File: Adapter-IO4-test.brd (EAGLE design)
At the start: 22 parts, among them CON1 CONNECTOR-IO4INV

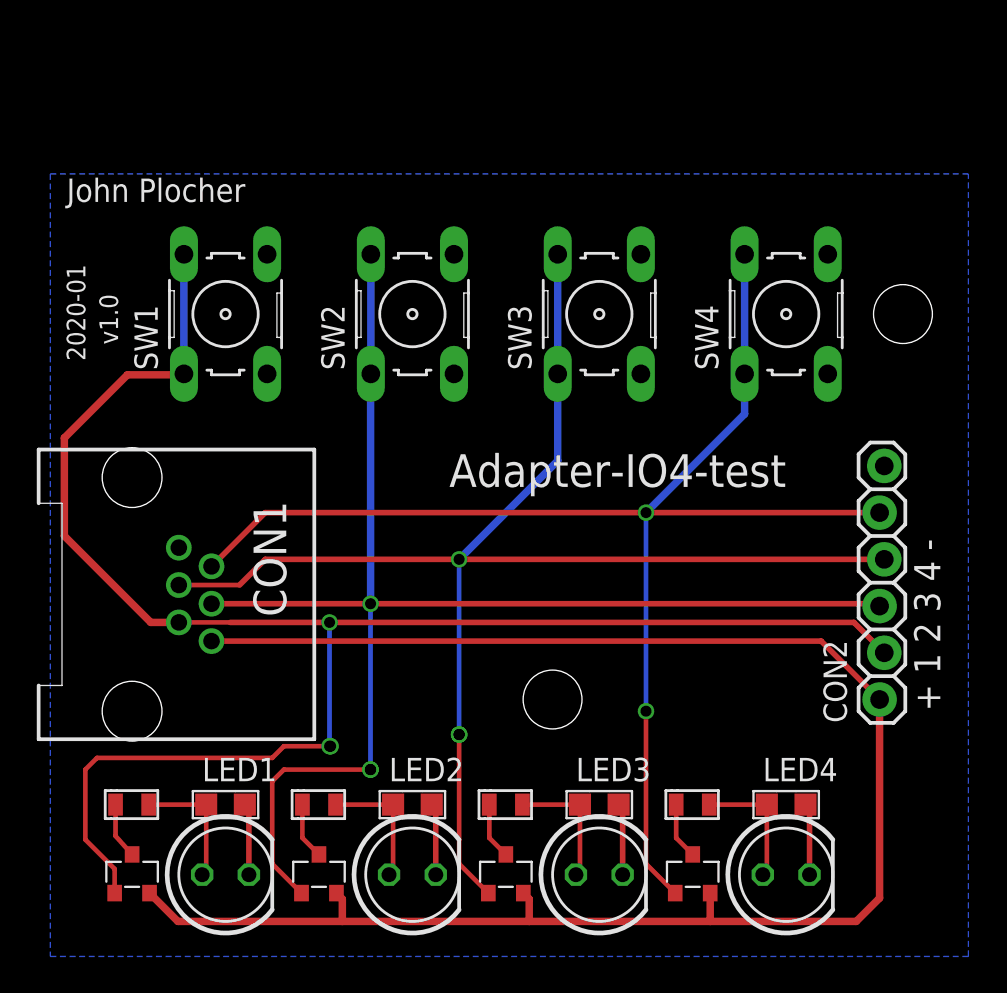
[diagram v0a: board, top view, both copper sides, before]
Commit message: simplified design
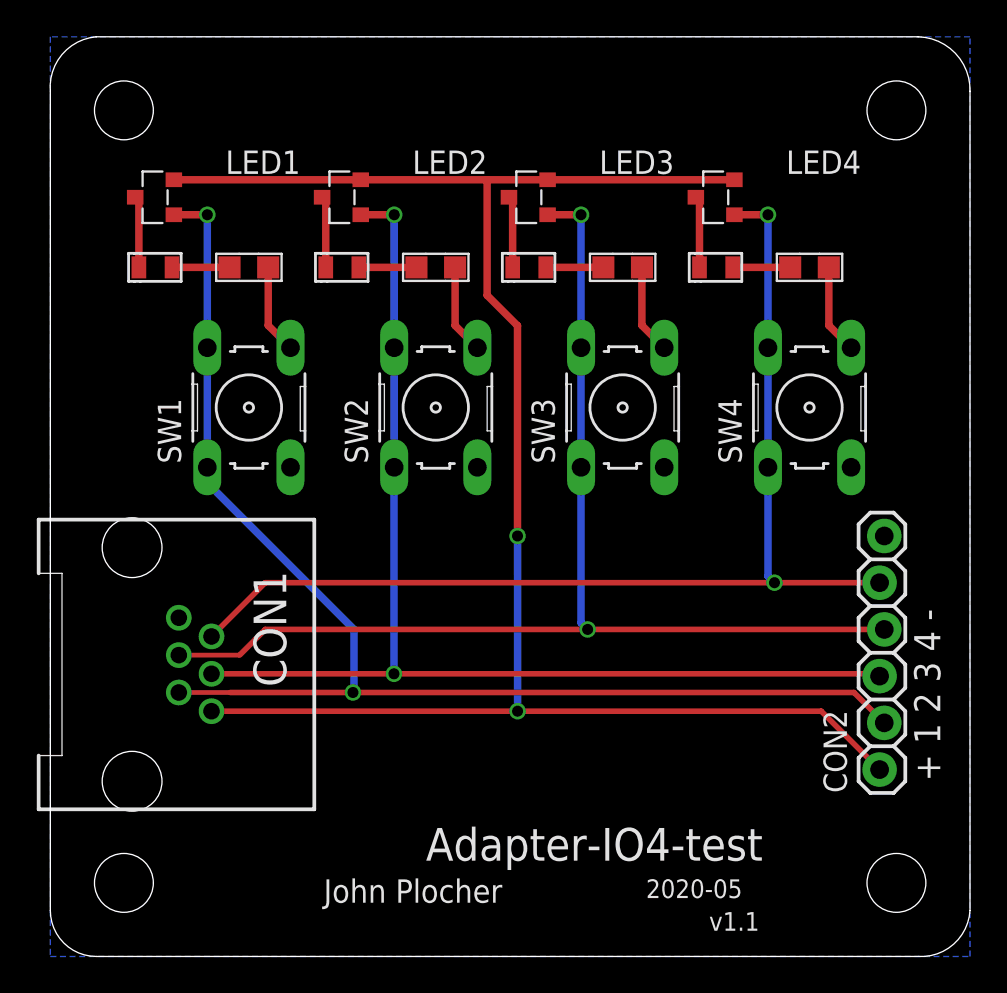
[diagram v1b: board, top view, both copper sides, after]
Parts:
- removed LED5, LED6, LED7, LED8: (no value), SPCoast:LED5MM
- added BOARD1: BOARD50X50-NOHOLES, SPCoast:BOARD-SEEED5X5-NOHOLES
- moved Q1 36.9 mm to (5.71, 41.3), turned to 90 degrees
- moved Q2 36.9 mm to (15.9, 41.3), turned to 90 degrees
- moved Q3 36.9 mm to (26.0, 41.3), turned to 90 degrees
- moved Q4 36.9 mm to (36.2, 41.3), turned to 90 degrees
- moved LED1 29.2 mm to (10.8, 37.5)
- moved LED2 29.2 mm to (21.0, 37.5)
- moved LED3 29.2 mm to (31.1, 37.5)
- moved LED4 29.2 mm to (41.3, 37.5)
- moved R1 29.2 mm to (5.71, 37.5)
- moved R2 29.2 mm to (15.9, 37.5)
- moved R3 29.2 mm to (26.0, 37.5)
- moved R4 29.2 mm to (36.2, 37.5)
- moved SW1 5.24 mm to (10.8, 29.8)
- moved SW2 5.24 mm to (21.0, 29.8)
- moved SW3 5.24 mm to (31.1, 29.8)
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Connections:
- net GND: no longer LED5.K, LED6.K, LED7.K, LED8.K
- net N$16: no longer LED8.A
- net N$2: no longer LED5.A
- net N$4: no longer LED6.A
- net N$6: no longer LED7.A
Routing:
- net N$7: track 95.0 -> 70.2 mm
- net N$10: track 75.1 -> 59.5 mm
- net N$8: track 76.7 -> 63.1 mm, vias 3 -> 2
- net N$9: track 76.5 -> 63.4 mm, vias 3 -> 2
- net N$6: track 7.03 -> 3.13 mm
- net N$4: track 7.03 -> 3.13 mm
- net N$2: track 7.03 -> 3.13 mm
- net N$16: track 7.03 -> 3.13 mm
- net GND: track 15.6 -> 19.5 mm
- net VCC: track 94.2 -> 97.7 mm, vias 0 -> 2
- net N$1: track 3.05 -> 3.89 mm
- net N$15: track 3.08 -> 3.89 mm
- net N$5: track 3.08 -> 3.89 mm
- net N$3: track 3.08 -> 3.89 mm
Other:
- board outline added: 50 x 50 mm
- board text added: "2020-05"
- board text added: "v1.1"
- board text removed: "2020-01"
- board text removed: "v1.0"
